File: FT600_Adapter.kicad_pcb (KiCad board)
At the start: 4 copper layers, 39 x 53 mm, 39 parts, among them J1 692622030100, J2 Conn_02x20_Odd_Even, U1 FT600Q-T, Y1 30MHz

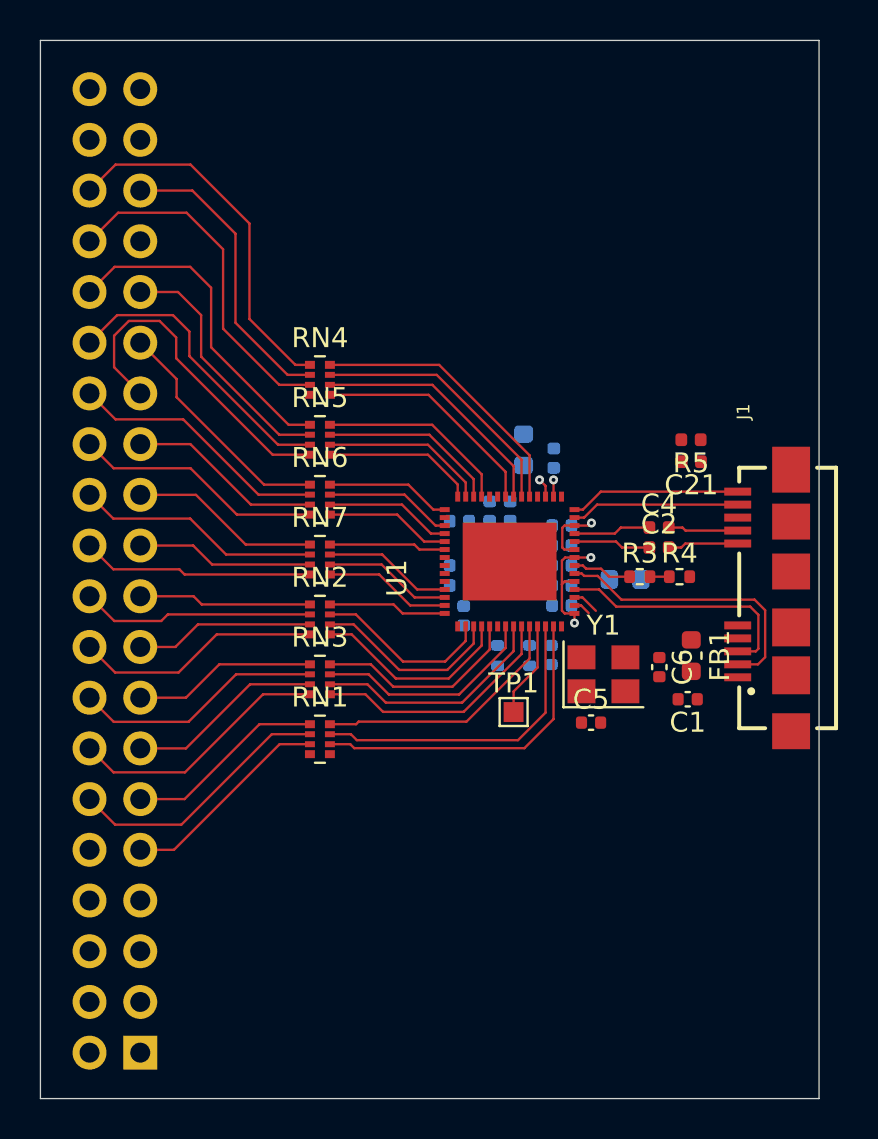
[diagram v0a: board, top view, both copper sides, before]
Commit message: Updated PCB layout
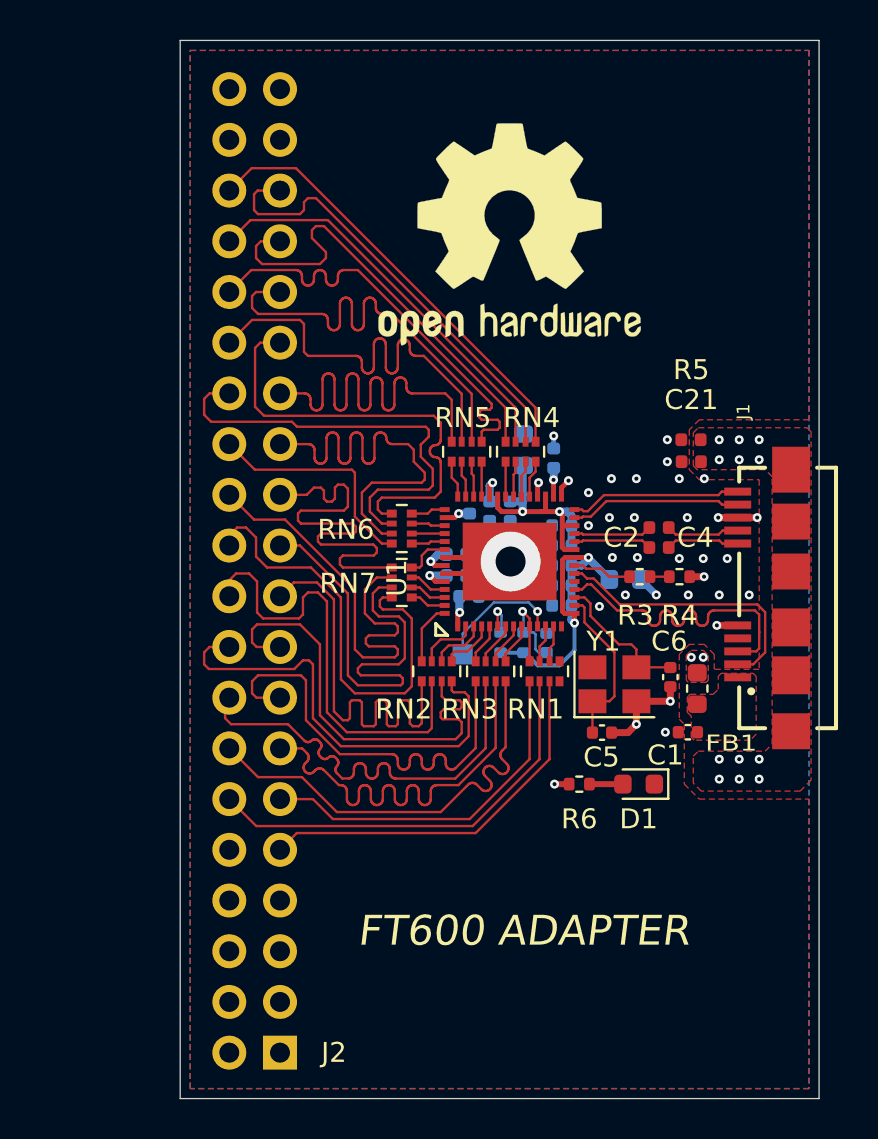
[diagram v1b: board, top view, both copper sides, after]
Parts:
- added D1: GREEN, LED_SMD:LED_0603_1608Metric, F.Cu at (130.0, 114.2)
- added R6: 10K, Resistor_SMD:R_0402_1005Metric, F.Cu at (127.0, 114.2)
- added REF**: OSHW-Logo2_14.6x12mm_SilkScreen, Symbol:OSHW-Logo2_14.6x12mm_SilkScreen, F.Cu at (123.5, 86.7)
- TP1: moved to B.Cu
- moved RN1 11.8 mm to (125.2, 108.6), turned to 90 degrees
- moved RN4 10.7 mm to (124.0, 97.6), turned to 270 degrees
- moved RN3 8.56 mm to (122.5, 108.6), turned to 90 degrees
- moved RN5 7.37 mm to (121.3, 97.6), turned to 270 degrees
- moved J2 7.00 mm to (112.0, 127.7)
- moved RN2 6.40 mm to (119.8, 108.6), turned to 90 degrees
- moved RN6 4.35 mm to (118.1, 101.5)
- moved RN7 4.26 mm to (118.1, 104.2)
- moved TP1 3.85 mm to (121.2, 107.8)
- moved FB1 1.68 mm to (132.9, 109.5)
- moved C1 1.65 mm to (132.4, 111.7)
- moved C12 1.00 mm to (121.5, 104.8), turned to 0 degrees
- moved C6 0.74 mm to (131.6, 108.9)
- moved Y1 0.74 mm to (128.8, 109.2)
- moved C5 0.74 mm to (128.1, 111.7)
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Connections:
- net Net-(C1-Pad1) renamed /CONN_VBUS
- J1 pad S1: Net-(J1-PadS1) -> /SHIELD
- J1 pad S2: Net-(J1-PadS2) -> /SHIELD
- J1 pad S3: Net-(J1-PadS3) -> /SHIELD
- J1 pad S4: Net-(J1-PadS4) -> /SHIELD
- J1 pad S5: Net-(J1-PadS5) -> /SHIELD
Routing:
- net +3V3: track 6.71 -> 68.7 mm, vias 3 -> 6
- net +5V: track 0.00 -> 22.6 mm, vias 0 -> 1
- net /FPGA_D3: track 0.00 -> 22.6 mm
- net +1V0: track 4.17 -> 26.5 mm, vias 2 -> 4
- net GND: track 0.00 -> 18.0 mm, vias 0 -> 32
- net VBUS: track 0.00 -> 16.2 mm, vias 0 -> 3
- net /FTDI_GPIO1: track 16.5 -> 1.83 mm
- net /FTDI_GPIO0: track 15.8 -> 1.87 mm
- net /FPGA_D15: track 8.67 -> 22.5 mm
- net /FPGA_BE1: track 8.97 -> 22.6 mm
- net /FPGA_D13: track 8.89 -> 22.4 mm
- net /FPGA_RXFN: track 9.19 -> 22.6 mm
- net /FPGA_D11: track 9.53 -> 22.5 mm
- net /FPGA_D9: track 9.76 -> 22.5 mm
- net /FPGA_RDN: track 9.83 -> 22.5 mm
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- added copper zone on F.Cu, net /CONN_VBUS
- added copper zone on F.Cu, net /SHIELD
- added copper zone on B.Cu, net GND
- added copper zone on F.Cu, net GND
- added copper zone on In1.Cu, net GND
- added copper zone on In2.Cu, net GND
- added copper zone on F.Cu, net VBUS
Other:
- board size 39 x 53 mm -> 32 x 53 mm
- net class GND: trace_width 0.35 -> 0.25
- net class Outer_Impedance_50_90 added: clearance 0.15, trace_width 0.12, via_dia 0.45, via_drill 0.2
- board text added: "FT600 ADAPTER"
